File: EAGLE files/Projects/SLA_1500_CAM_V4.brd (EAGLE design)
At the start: 37.8 x 26.4 mm, 88 parts, among them J2 JST GH SM06B, J3 MOLEX 53261-03, J4 MOLEX 53261-04, J5 MOLEX 53261-04, J6 MOLEX 53261-04, U11 TXS0102, U2 TPS73633DCQR, U8 TXS0102, U9 TXS0102

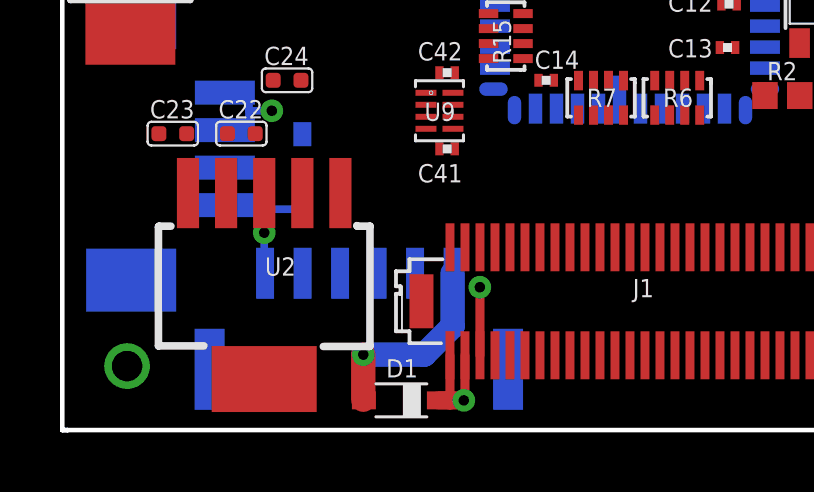
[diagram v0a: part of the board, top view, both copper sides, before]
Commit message: Update SLA1500 CAM
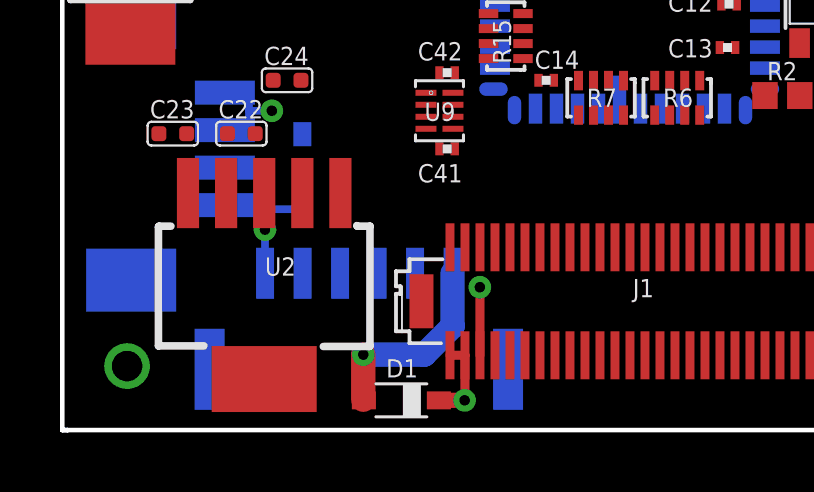
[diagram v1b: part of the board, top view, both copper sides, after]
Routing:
- net P5V: track 3.85 -> 2.87 mm
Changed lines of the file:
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@@
 </polygon>
 <wire x1="-12.7" y1="-5.217" x2="-13.502" y2="-5.217" width="0.254" layer="16"/>
-<wire x1="-12.164" y1="-9.988" x2="-12.192" y2="-9.988" width="0.254" layer="16"/>
-<wire x1="-12.192" y1="-9.988" x2="-12.192" y2="-8.636" width="0.254" layer="16"/>
-<via x="-12.192" y="-8.636" extent="15-16" drill="0.35"/>
+<wire x1="-12.164" y1="-9.988" x2="-12.1666" y2="-9.988" width="0.254" layer="16"/>
+<wire x1="-12.1666" y1="-9.988" x2="-12.1666" y2="-8.5344" width="0.254" layer="16"/>
+<via x="-12.1666" y="-8.5344" extent="15-16" drill="0.35"/>
 <wire x1="-13.502" y1="-3.967" x2="-12.797" y2="-3.967" width="0.254" layer="16"/>
 <wire x1="-12.797" y1="-3.967" x2="-12.7" y2="-4.064" width="0.254" layer="16"/>
@@
 <wire x1="-11.8925" y1="-3.556" x2="-12.7" y2="-4.064" width="0" layer="19" extent="1-16"/>
 <wire x1="-14.7775" y1="-5.334" x2="-13.502" y2="-5.217" width="0" layer="19" extent="1-16"/>
-<wire x1="-12.192" y1="-7.314" x2="-12.192" y2="-8.636" width="0" layer="19" extent="1-16"/>
+<wire x1="-12.192" y1="-7.314" x2="-12.1666" y2="-8.5344" width="0" layer="19" extent="1-16"/>
 <wire x1="14.6812" y1="9.4742" x2="16.764" y2="9.017" width="0" layer="19" extent="1-1"/>
 <wire x1="14.6812" y1="7.6962" x2="14.6812" y2="9.4742" width="0" layer="19" extent="1-1"/>
@@
 <vertex x="-19.0754" y="6.096"/>
 </polygon>
-<wire x1="-6.37" y1="-14.224" x2="-5.9944" y2="-14.224" width="0.6096" layer="1"/>
-<via x="-5.5372" y="-14.224" extent="1-2" drill="0.35"/>
-<wire x1="-5.9944" y1="-14.224" x2="-5.5372" y2="-14.224" width="0.6096" layer="1"/>
-<wire x1="-6" y1="-12.722" x2="-6" y2="-14.2184" width="0.3048" layer="1"/>
-<wire x1="-6" y1="-14.2184" x2="-5.9944" y2="-14.224" width="0.3048" layer="1"/>
-<wire x1="-5.5" y1="-12.722" x2="-5.5" y2="-14.1868" width="0.3048" layer="1"/>
-<wire x1="-5.5" y1="-14.1868" x2="-5.5372" y2="-14.224" width="0.3048" layer="1"/>
+<wire x1="-5.5" y1="-12.722" x2="-6" y2="-12.722" width="0.3048" layer="1"/>
+<wire x1="-6.37" y1="-14.224" x2="-5.5118" y2="-14.224" width="0.508" layer="1"/>
+<via x="-5.5118" y="-14.224" extent="1-2" drill="0.35"/>
+<wire x1="-5.5" y1="-12.722" x2="-5.5" y2="-14.2122" width="0.3048" layer="1"/>
+<wire x1="-5.5" y1="-14.2122" x2="-5.5118" y2="-14.224" width="0.3048" layer="1"/>
 <wire x1="-17.614" y1="3.556" x2="1.2192" y2="24.4602" width="0" layer="19" extent="16-16"/>
 <wire x1="-17.526" y1="1.27" x2="-17.614" y2="3.556" width="0" layer="19" extent="16-16"/>
